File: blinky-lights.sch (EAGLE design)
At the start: 20 parts, among them Q1 NFET, U1 555, U2 A2678EAT

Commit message: board layout
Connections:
- new net SENSE: LED1.C, Q1.G, R4.1
- net FEEDBACK: no longer LED1.C, Q1.G, R4.1
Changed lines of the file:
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@@
 <net name="FEEDBACK" class="0">
-<segment>
-<pinref part="LED1" gate="G$1" pin="C"/>
-<wire x1="218.44" y1="106.68" x2="215.9" y2="106.68" width="0.1524" layer="91"/>
-<wire x1="215.9" y1="106.68" x2="215.9" y2="104.14" width="0.1524" layer="91"/>
-<pinref part="R4" gate="G$1" pin="1"/>
-<wire x1="200.66" y1="104.14" x2="215.9" y2="104.14" width="0.1524" layer="91"/>
-<wire x1="200.66" y1="104.14" x2="200.66" y2="132.08" width="0.1524" layer="91"/>
-<junction x="200.66" y="104.14"/>
-<pinref part="Q1" gate="G$1" pin="G"/>
-</segment>
 <segment>
 <pinref part="U2" gate="G$1" pin="DATA"/>
@@
 </segment>
 </net>
+<net name="SENSE" class="0">
+<segment>
+<pinref part="LED1" gate="G$1" pin="C"/>
+<wire x1="218.44" y1="106.68" x2="215.9" y2="106.68" width="0.1524" layer="91"/>
+<wire x1="215.9" y1="106.68" x2="215.9" y2="104.14" width="0.1524" layer="91"/>
+<pinref part="R4" gate="G$1" pin="1"/>
+<wire x1="200.66" y1="104.14" x2="215.9" y2="104.14" width="0.1524" layer="91"/>
+<wire x1="200.66" y1="104.14" x2="200.66" y2="132.08" width="0.1524" layer="91"/>
+<junction x="200.66" y="104.14"/>
+<pinref part="Q1" gate="G$1" pin="G"/>
+</segment>
+</net>
 </nets>
 </sheet>
 </sheets>
+<errors>
+</errors>
 </schematic>
 </drawing>

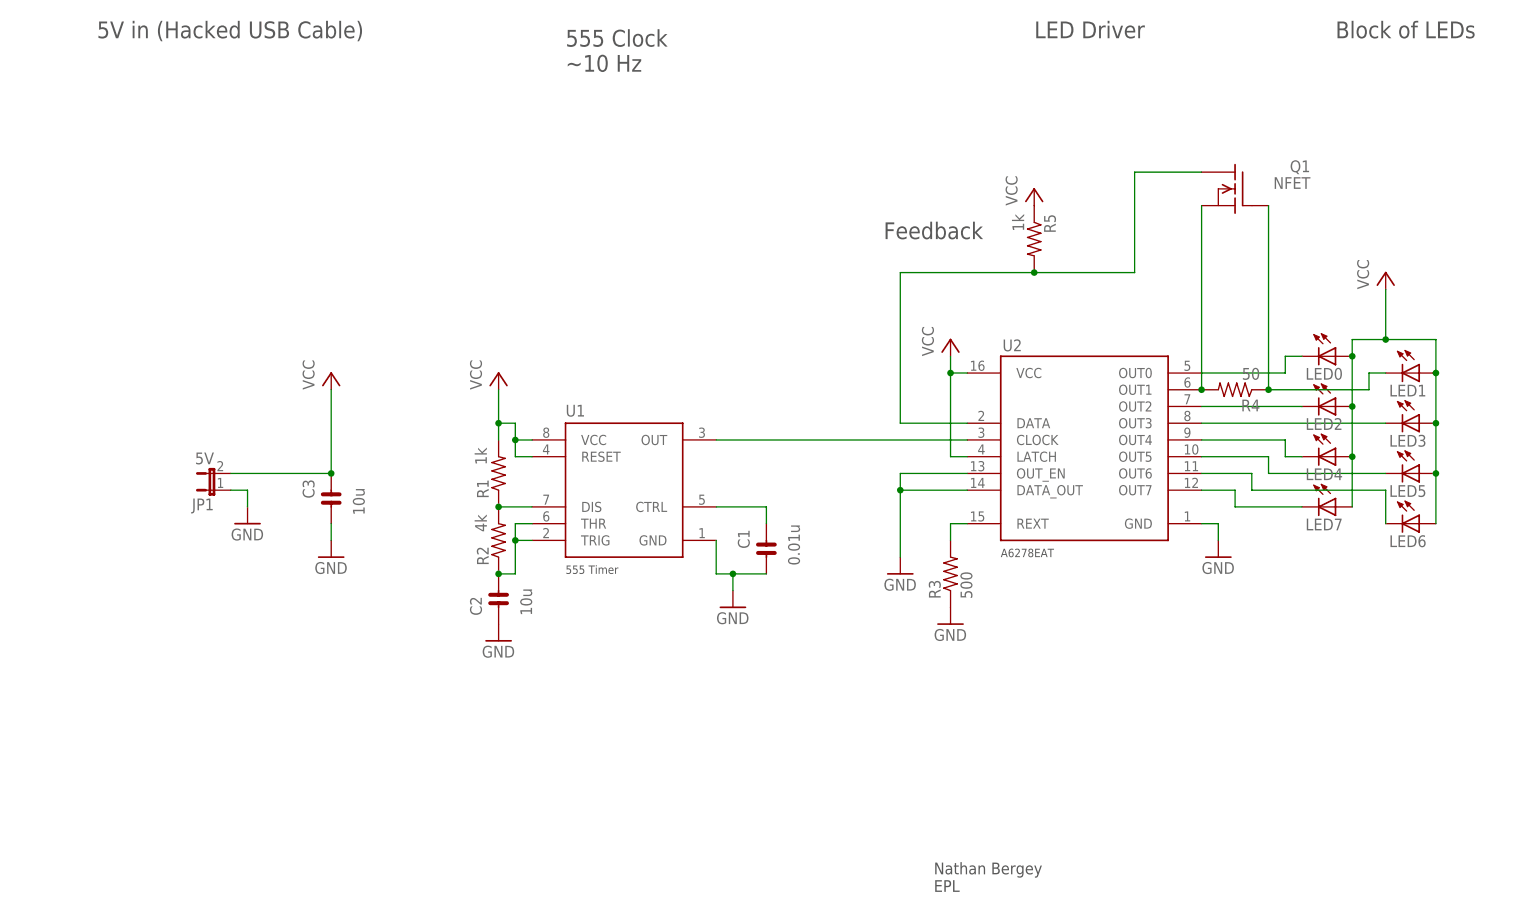
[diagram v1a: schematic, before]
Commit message: schematic and board clean up
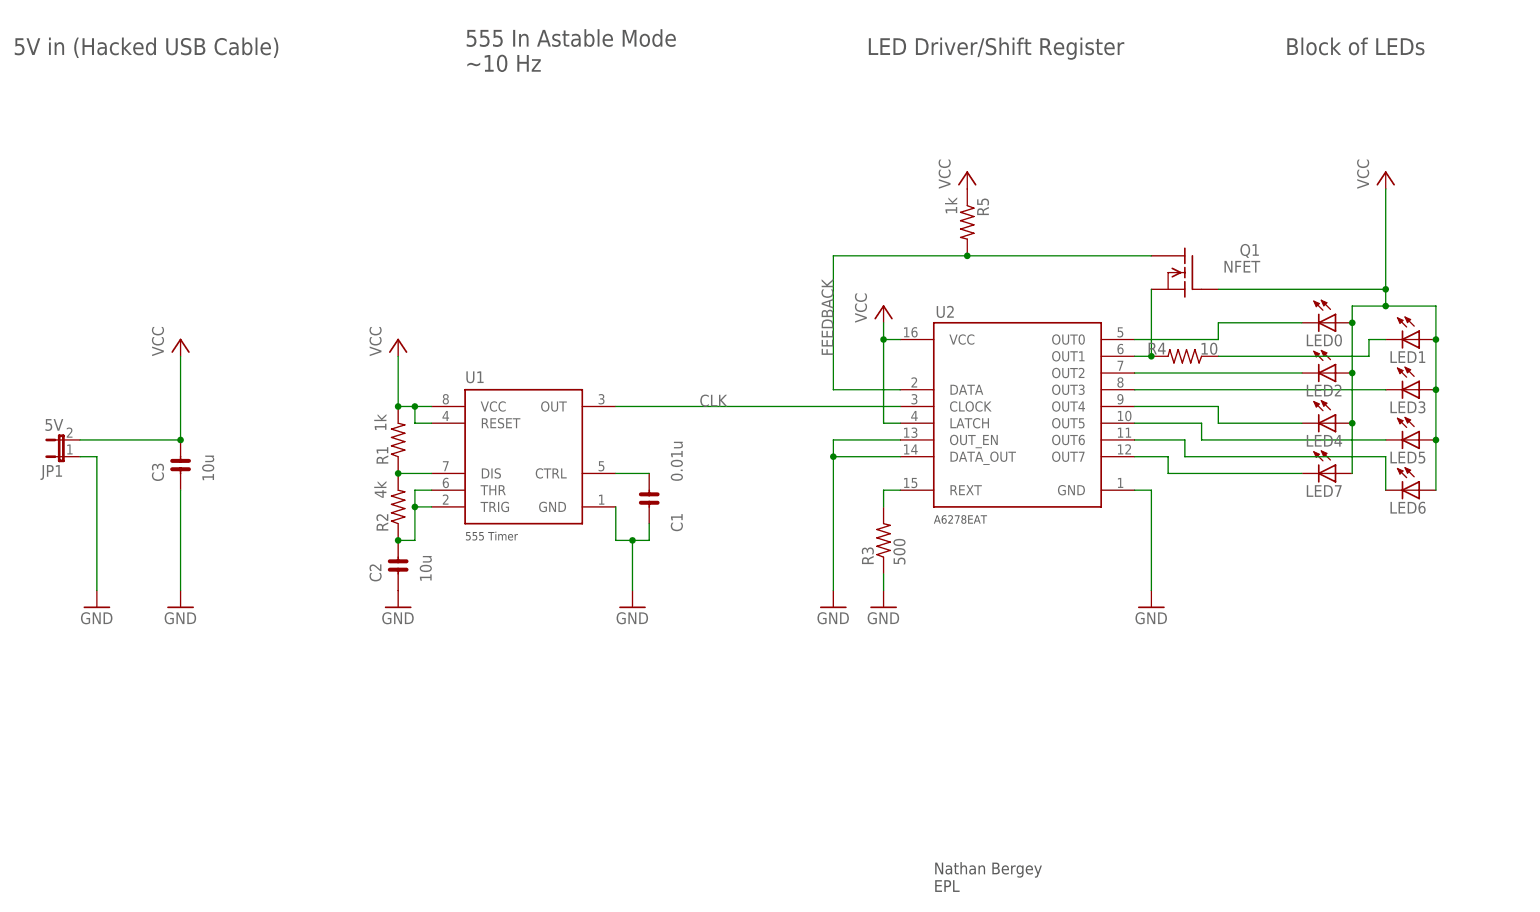
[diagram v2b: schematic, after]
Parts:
- R4: value 50 -> 10
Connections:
- net SENSE: no longer Q1.G
- net VCC: now also Q1.G
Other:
- note added: "555 In Astable Mode ~10 Hz"
- note added: "LED Driver/Shift Register"
- note removed: "555 Clock ~10 Hz"
- note removed: "Feedback"
- note removed: "LED Driver"
- moved on the sheet: C1, C2, C3, JP1, LED0, LED1, LED2, LED3, LED4, LED5, LED6, LED7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
